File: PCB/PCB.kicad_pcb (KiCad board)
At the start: 2 copper layers, 130 x 120 mm, 47 parts, among them J1 Conn_01x08_Pin, J2 Conn_01x04_Socket, SW1 SW_Push, SW10 SW_Push, SW11 SW_Push, SW12 SW_Push, SW13 RotaryEncoder_Switch, SW14 RotaryEncoder_Switch, SW15 RotaryEncoder_Switch, SW16 RotaryEncoder_Switch, SW17 RotaryEncoder_Switch, SW18 RotaryEncoder_Switch, SW2 SW_Push, SW3 SW_Push, SW4 SW_Push, SW5 SW_Push, SW6 SW_Push, SW7 SW_Push, SW8 SW_Push, SW9 SW_Push, U1 MCP23017x-x-SO

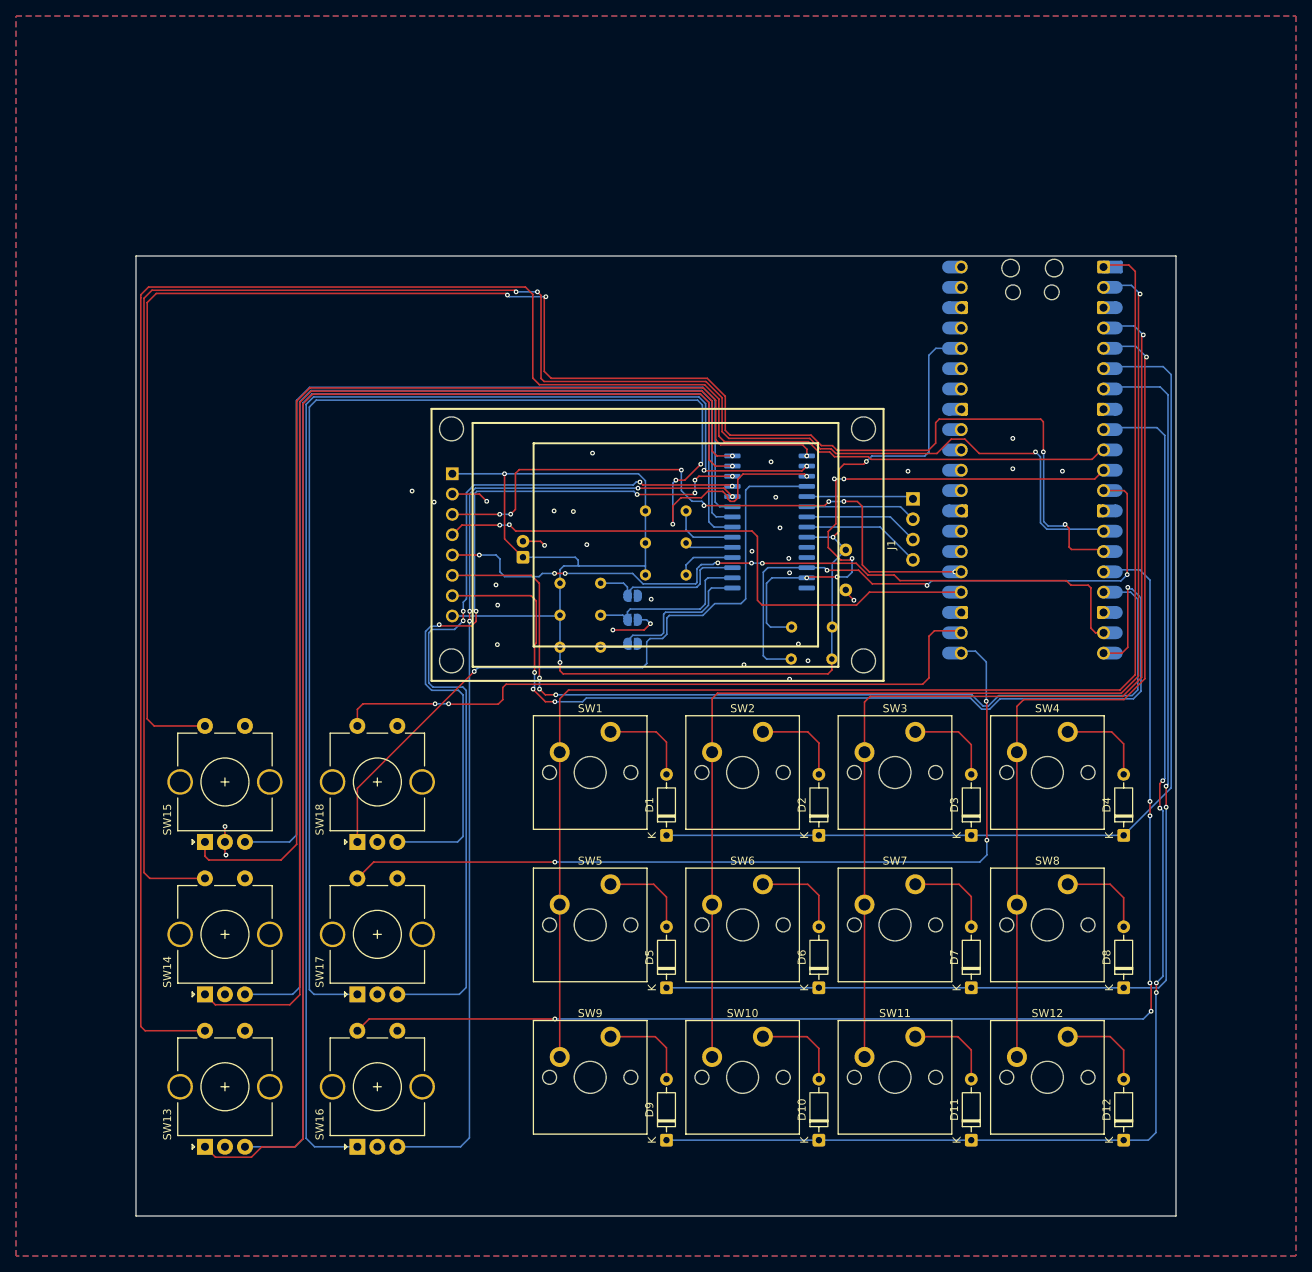
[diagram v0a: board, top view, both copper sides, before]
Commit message: added CAD/PCB.step
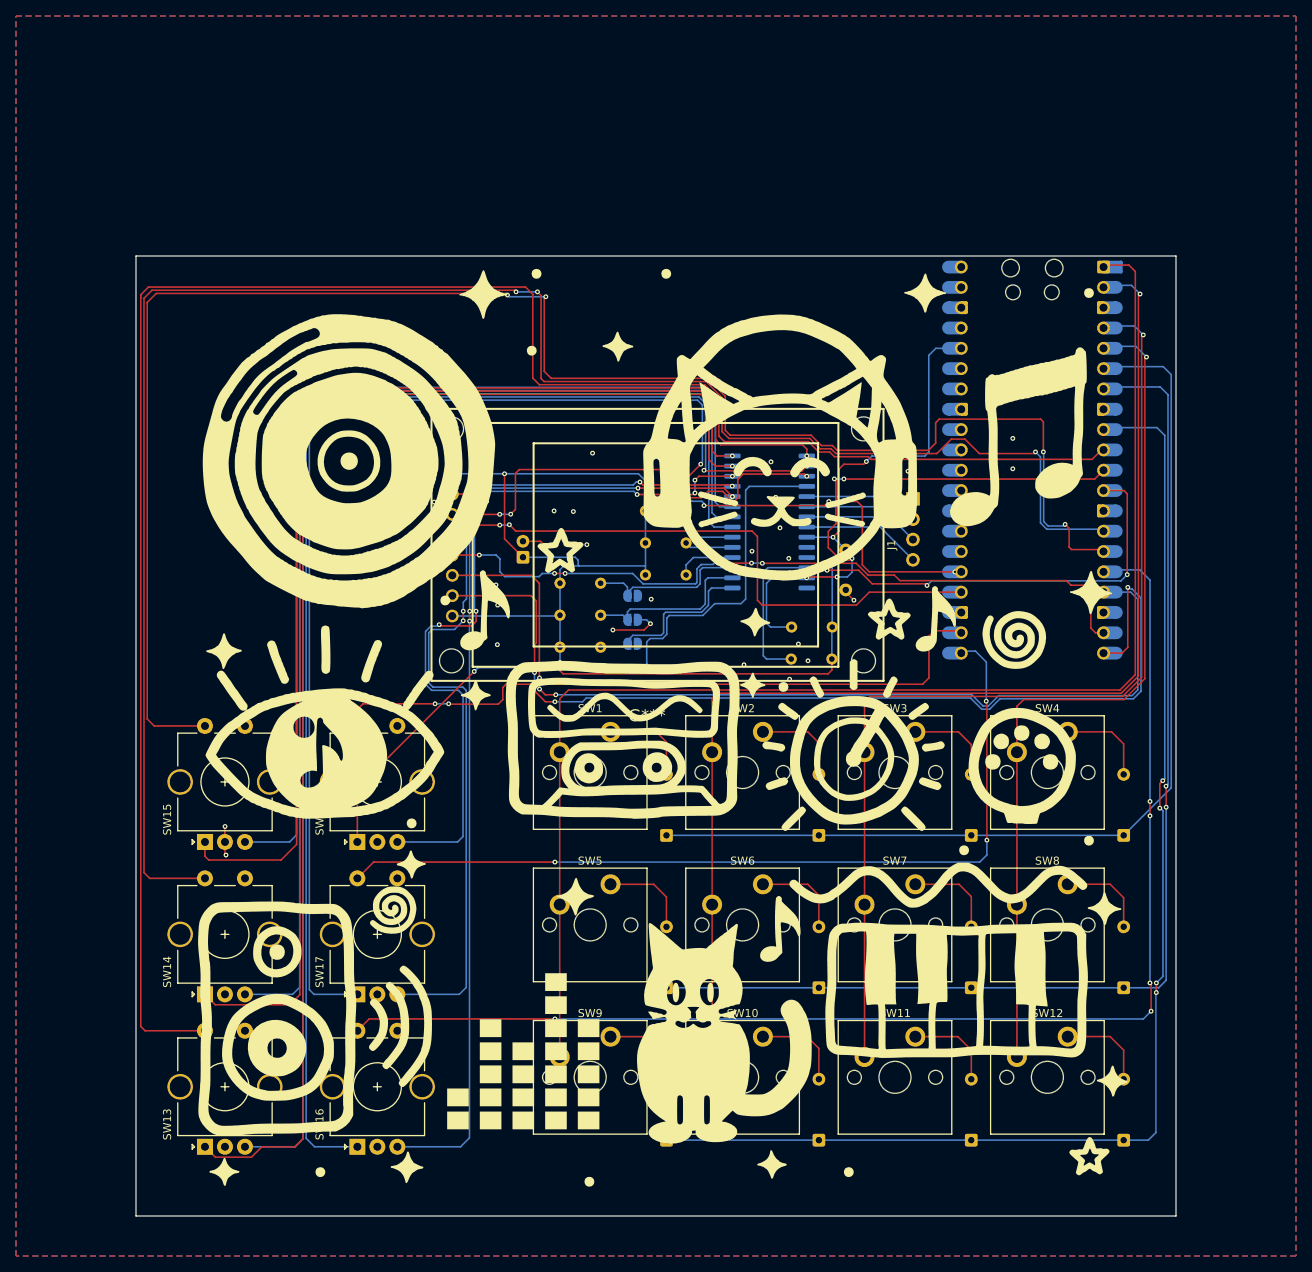
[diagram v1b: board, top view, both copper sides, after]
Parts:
- added G***: LOGO, LOGO, F.Cu at (143.9, 112.5)
- D1, D10, D11, D12, D2, D3, D4, D5, D6, D7, D8, D9: moved to B.Cu
